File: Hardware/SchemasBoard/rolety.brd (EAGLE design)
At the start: 46.7 x 22.9 mm, 30 parts, among them IC1 LNK304, IC2 MCP1703DB, K1 FRS1B, K2 FRS1B, T1 BC846, T2 BC846

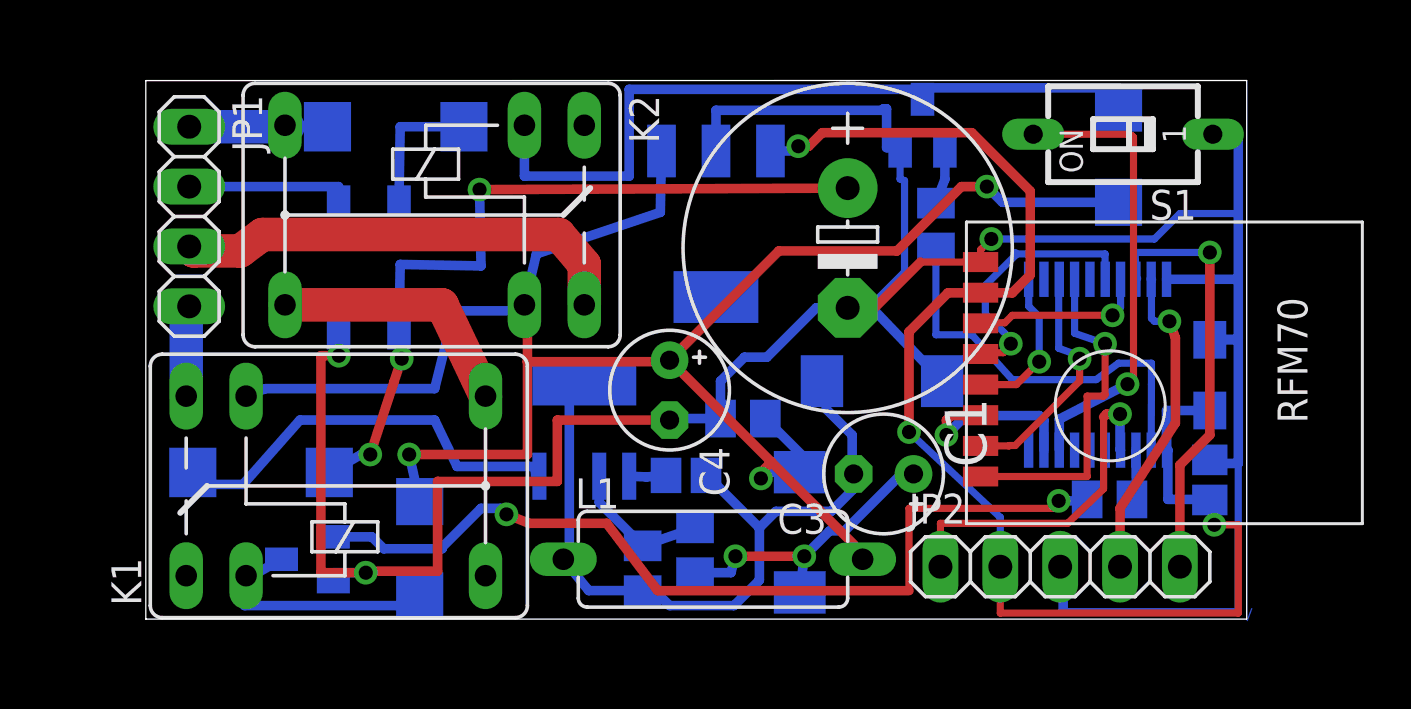
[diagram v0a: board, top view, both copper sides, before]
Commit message: a
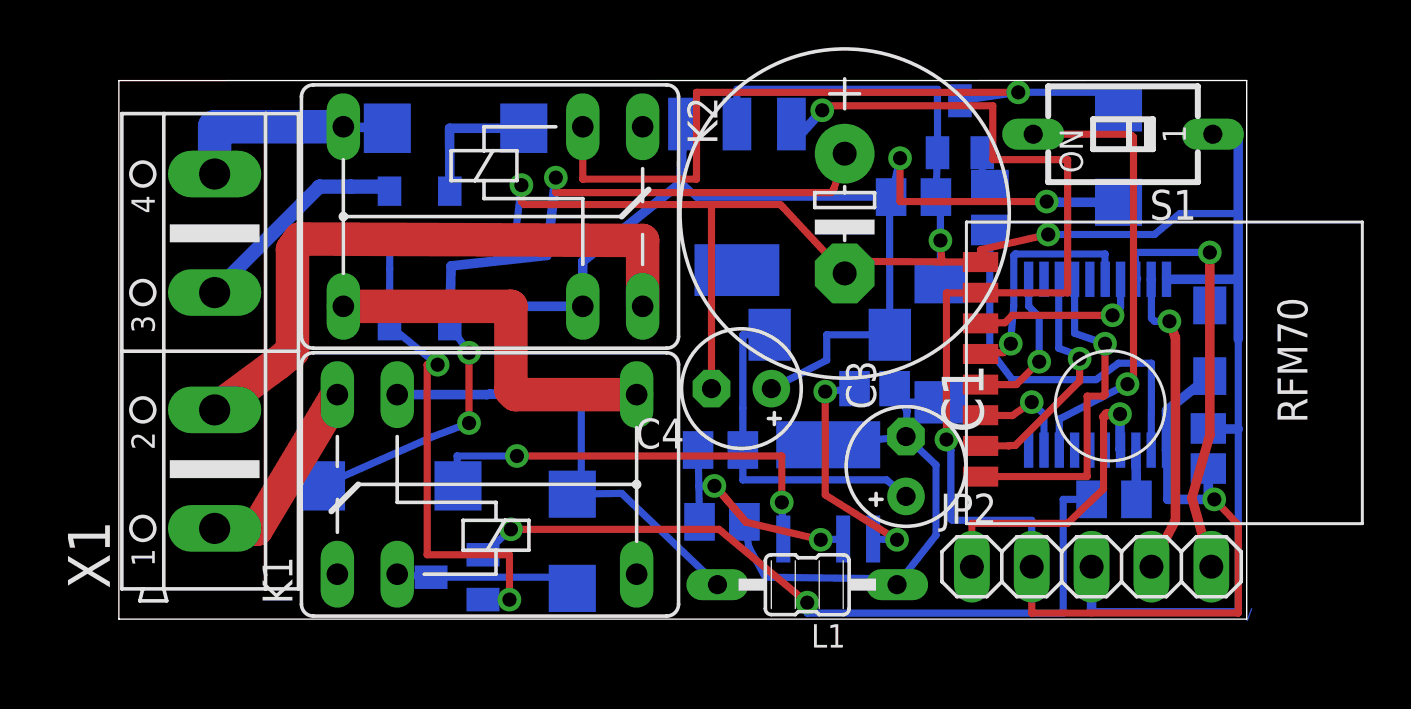
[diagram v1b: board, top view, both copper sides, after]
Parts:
- removed JP1: (no value), pinhead:1X04
- added X1: (no value), con-ptr500:AK500/4
- L1: value BC12 -> MMICC7; device inductors:BC12 -> inductors:MMICC7
- moved R7 11.9 mm to (32.6, 17.9), turned to 0 degrees
- moved IC1 10.7 mm to (29.0, 5.40)
- moved C2 8.81 mm to (30.9, 9.78)
- moved D4 8.48 mm to (29.0, 12.1), turned to 180 degrees
- moved D1 6.48 mm to (18.1, 3.30)
- moved K1 6.41 mm to (10.7, 5.71)
- moved T1 6.40 mm to (13.2, 1.78)
- moved R1 5.49 mm to (10.4, 5.65), turned to 180 degrees
- moved R3 4.39 mm to (24.4, 7.18), turned to 0 degrees
- moved L1 4.14 mm to (28.1, 1.46), turned to 180 degrees
- moved R4 3.90 mm to (24.4, 4.13), turned to 180 degrees
- moved C4 3.05 mm to (25.3, 9.78), turned to 180 degrees
- moved D3 2.98 mm to (33.7, 11.7), turned to 90 degrees
- moved R2 2.54 mm to (13.1, 20.8)
- moved K2 2.48 mm to (18.5, 17.1)
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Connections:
- net N$36: now also X1.4; no longer JP1.1
- net N$4: now also X1.3; no longer JP1.2
- net N$7: now also X1.1; no longer JP1.4
- net N$8: now also X1.2; no longer JP1.3
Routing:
- net N$27: track 84.7 -> 71.5 mm, vias 3 -> 2
- net N$13: track 32.9 -> 22.8 mm
- net N$10: track 1.57 -> 10.2 mm, vias 0 -> 2
- net N$17: track 59.3 -> 66.5 mm
- net N$8: track 19.4 -> 26.3 mm
- net N$11: track 6.07 -> 12.0 mm, vias 0 -> 2
- net N$4: track 6.91 -> 12.6 mm
- net N$15: track 38.3 -> 32.6 mm
- net N$26: track 11.0 -> 16.1 mm
- net N$7: track 3.94 -> 8.44 mm
- net N$23: track 8.00 -> 4.60 mm
- net N$36: track 6.00 -> 9.34 mm
- net N$14: track 10.8 -> 7.72 mm
- net N$2: track 32.5 -> 35.2 mm
- net N$9: track 12.8 -> 14.5 mm, vias 2 -> 0
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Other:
- board size 46.7 x 22.9 mm -> 47.9 x 22.9 mm
